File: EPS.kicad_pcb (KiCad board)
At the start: 4 copper layers, 90.2 x 95.9 mm, 197 parts, among them IC1 BQ7791514PWR, IC10 INA260AIPWR, IC12 LM74700QDBVRQ1, IC13 LM74700QDBVRQ1, IC14 LM5176PWPR, IC15 SN65HVD1782QDRQ1, IC16 TPS2121RUXR, IC17 TCAN1046AVDRQ1, IC18 INA260AIPWR, IC19 LM5060Q1MM_NOPB, IC2 INA260AIPWR, IC20 LM5060Q1MM_NOPB, IC21 MCP2517FD-H_SL, IC3 INA260AIPWR, IC4 INA260AIPWR, IC5 TPS22990DMLR, IC6 TPS22990DMLR, IC7 TPS22990DMLR, IC9 INA260AIPWR, J1 Barrel_Jack_Switch, J2 PH1RA-02-UA, J3 WJ126V-5.0-2P, J4 USB_C_Receptacle_USB2.0_16P, J6 TagConnect_TC2030-NL, Q10 BSZ067N06LS3_G, Q11 BSZ067N06LS3_G, Q12 BSZ067N06LS3_G, Q13 BSZ067N06LS3_G, Q15 BSZ067N06LS3_G, Q16 BSZ067N06LS3_G, Q5 BSZ067N06LS3_G, Q6 BSZ067N06LS3_G, Q8 BSZ067N06LS3_G, Q9 BSZ067N06LS3_G, U2 RP2354A_60QFN, Y1 ABM8AIG-20MHz-12-2Z-T3, Y2 ABM8-272-T3

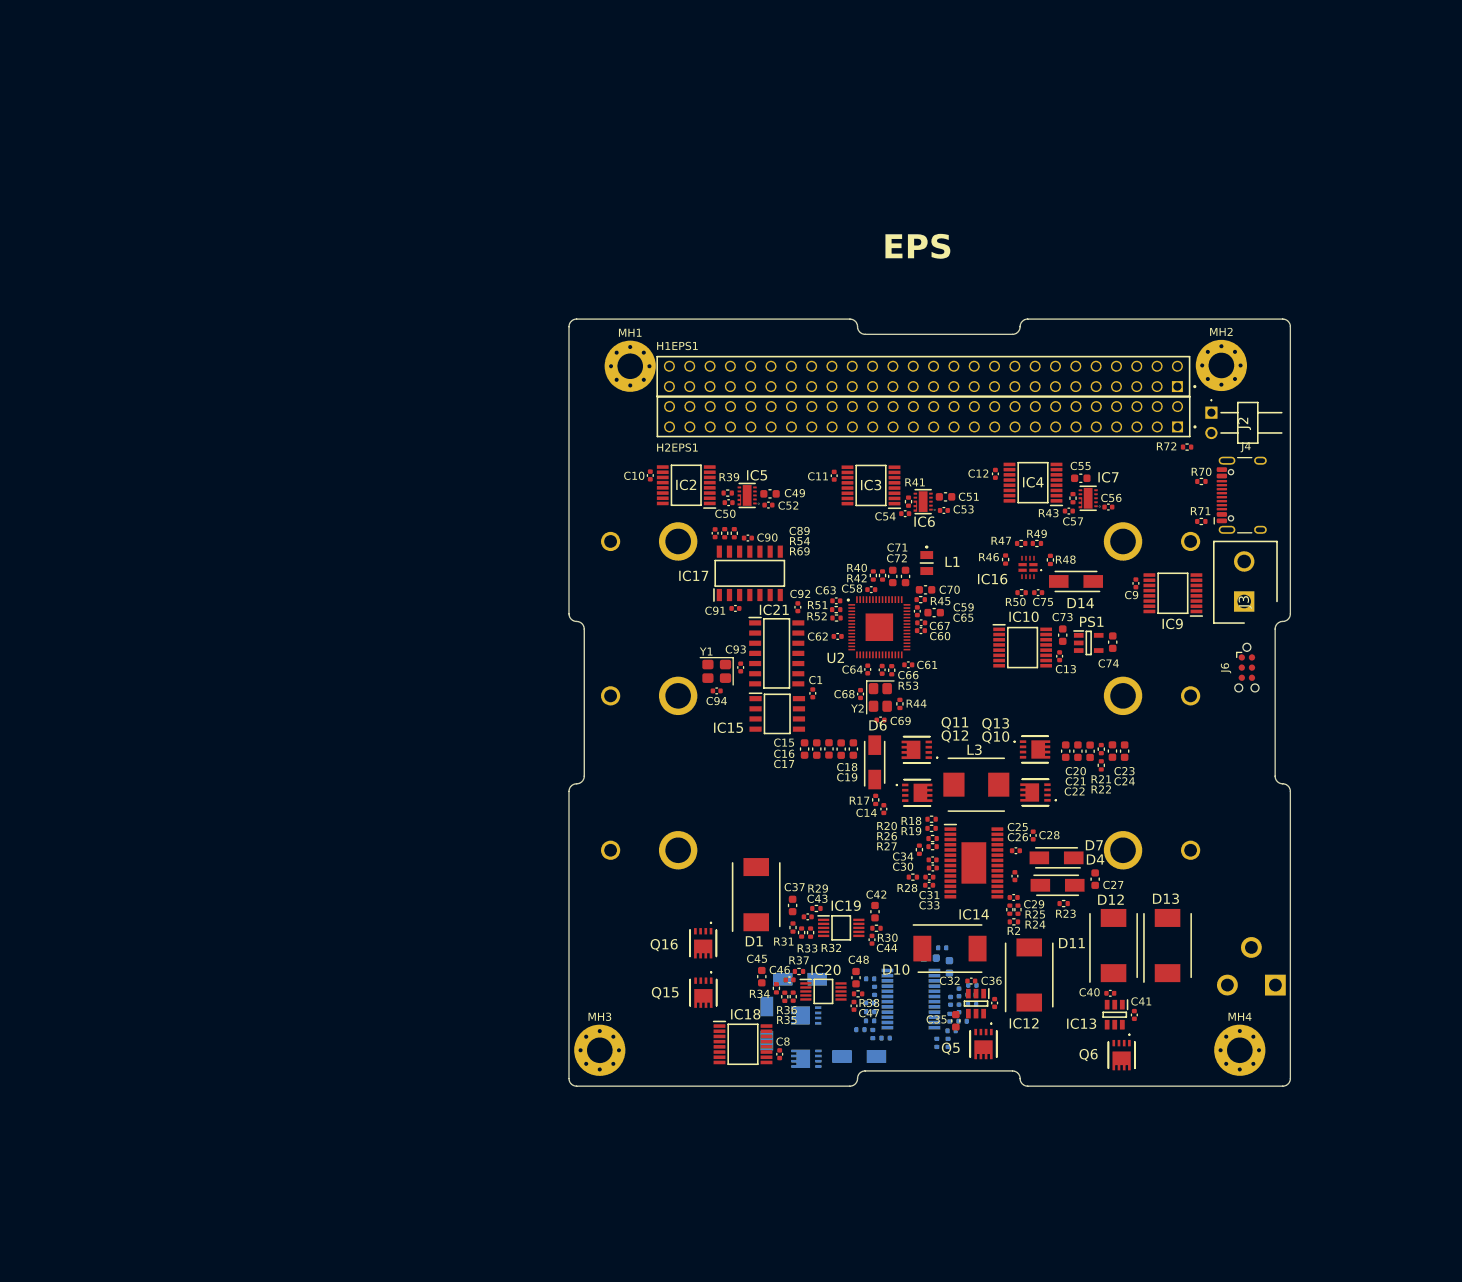
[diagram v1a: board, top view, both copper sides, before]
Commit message: Rev 1 version
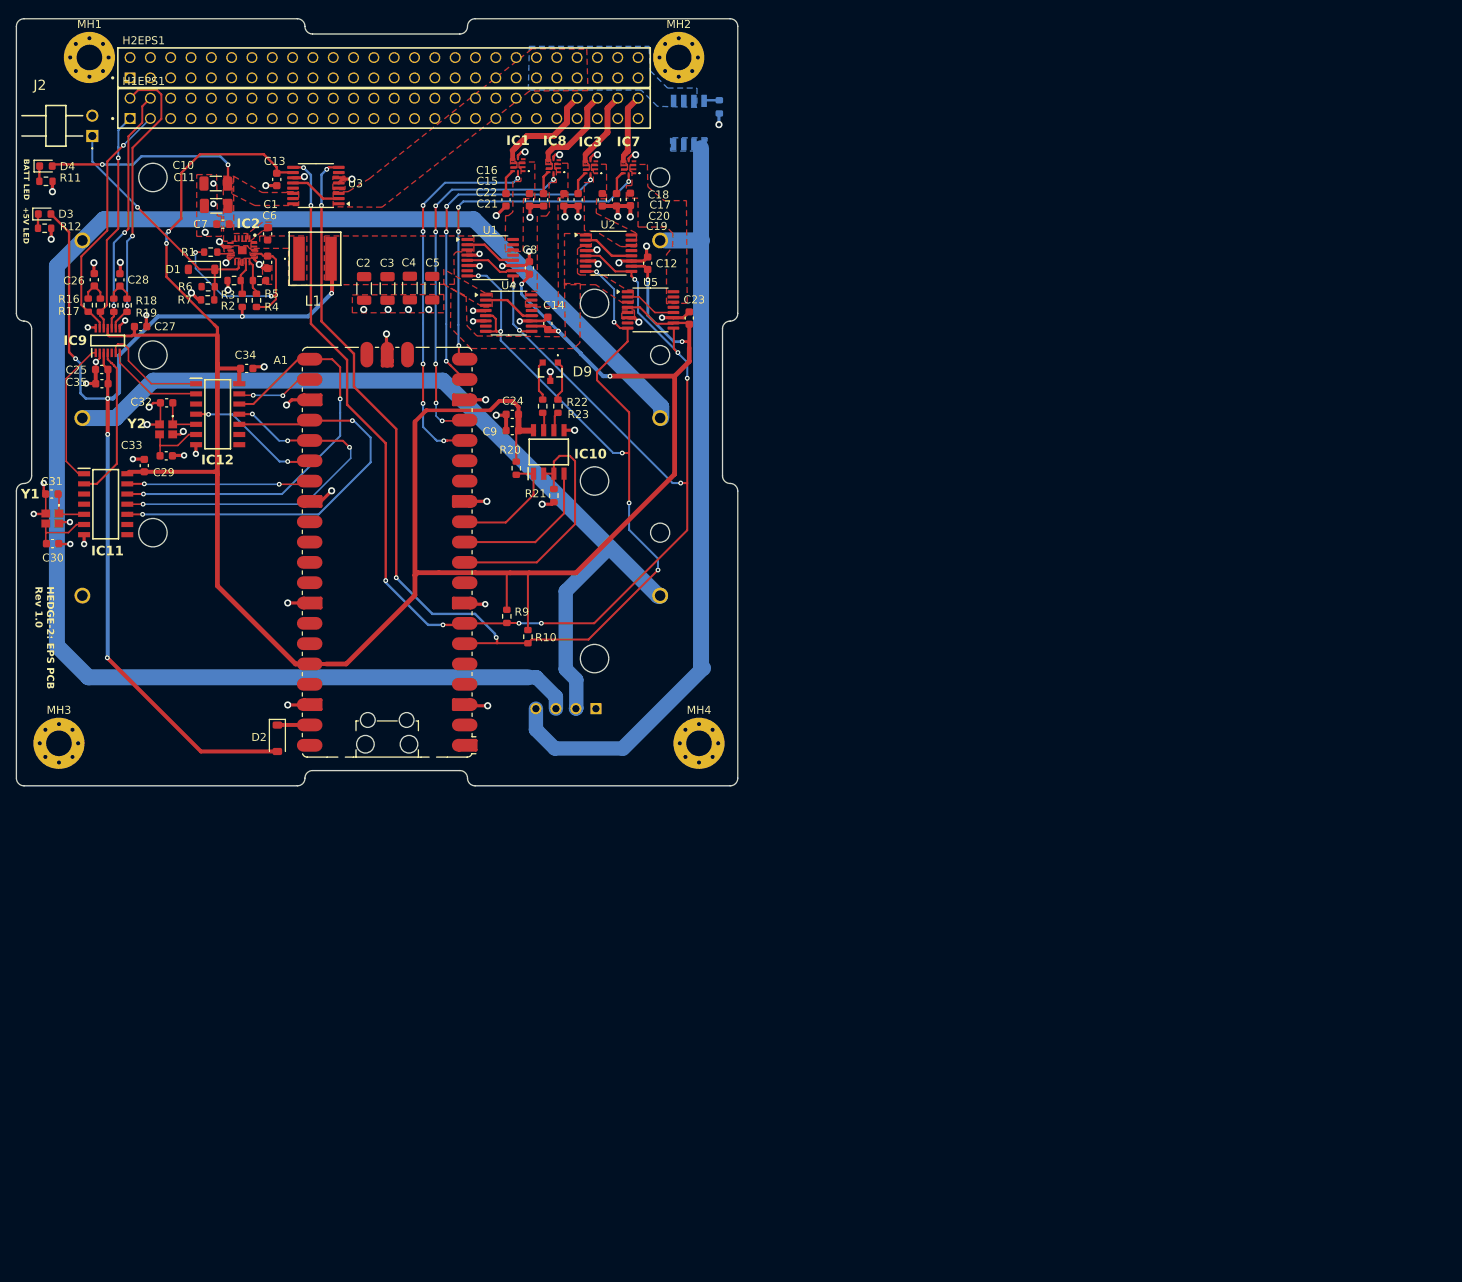
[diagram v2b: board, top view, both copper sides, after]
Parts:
- removed C36, C41, C43, C44, C46, C47, C50, C54, C57, C58, C59, C60, C61, C62, C63, C64, C66, C67, C75, C89, C90, C91, C92: 100n, Capacitor_SMD:C_0402_1005Metric
- removed C37, C42, C45, C48: 22u, Capacitor_SMD:C_0603_1608Metric
- removed C40: 22n, Capacitor_SMD:C_0402_1005Metric
- removed C49, C51, C55, C73, C74: 1u, Capacitor_SMD:C_0603_1608Metric
- removed C52, C53, C56: 220p, Capacitor_SMD:C_0402_1005Metric
- removed C65, C70, C71, C72: 4u7, Capacitor_SMD:C_0603_1608Metric
- removed C68, C69, C93, C94: 15p, Capacitor_SMD:C_0402_1005Metric
- removed D10, D11, D12, D13: SMCJ36A, HEDGE2:SMCJ36A
- removed D14, D5, D6, D7: CDBA240LL-HF, 40V 2A, HEDGE2:CDBA240LL-HF
- removed IC13: LM74700QDBVRQ1, HEDGE2:LM74700QDBVRQ1
- removed IC14: LM5176PWPR, HEDGE2:LM5176PWPR
- removed IC15: SN65HVD1782QDRQ1, HEDGE2:SN65HVD1782QDRQ1
- removed IC16: TPS2121RUXR, HEDGE2:TPS2121RUXR
- removed IC17: TCAN1046AVDRQ1, HEDGE2:TCAN1046AVDRQ1
- removed IC18, IC4: INA260AIPWR, HEDGE2:INA260AIPWR
- removed IC19, IC20: LM5060Q1MM_NOPB, HEDGE2:LM5060Q1MM_NOPB
- removed IC21: MCP2517FD-H_SL, HEDGE2:MCP2517FD-H_SL
- removed IC5, IC6: TPS22990DMLR, HEDGE2:TPS22990DMLR
- removed J3: WJ126V-5.0-2P, HEDGE2:WJ126V-5.0-2P
- removed J4: USB_C_Receptacle_USB2.0_16P, Connector_USB:USB_C_Receptacle_HCTL_HC-TYPE-C-16P-01A
- removed J6: TagConnect_TC2030-NL, Connector:Tag-Connect_TC2030-IDC-NL_2x03_P1.27mm_Vertical
- removed L3: 0630CDMCDDS-1R2MC, HEDGE2:0630CDMCDDS-1R2MC
- removed PS1: TLV75733PDBVR, HEDGE2:TLV75733PDBVR
- removed Q10, Q11, Q12, Q13, Q15, Q16, Q5, Q6, Q8, Q9: BSZ067N06LS3_G, HEDGE2:BSZ067N06LS3G
- removed R13: 450k, Resistor_SMD:R_0402_1005Metric
- removed R14, R30, R38: 100k, Resistor_SMD:R_0402_1005Metric
- removed R15, R39, R41, R43, R53, TH1: 10k, Resistor_SMD:R_0402_1005Metric
- removed R24, R25: 100, Resistor_SMD:R_0402_1005Metric
- removed R26: 93k1, Resistor_SMD:R_0402_1005Metric
- removed R27: 23k2, Resistor_SMD:R_0402_1005Metric
- removed R28: 7k5, Resistor_SMD:R_0402_1005Metric
- removed R29, R37: 9k09, Resistor_SMD:R_0402_1005Metric
- removed R31, R34: 200k, Resistor_SMD:R_0402_1005Metric
- removed R32, R35: 38k3, Resistor_SMD:R_0402_1005Metric
- removed R33, R36: 14k, Resistor_SMD:R_0402_1005Metric
- removed R40, R42: 27, Resistor_SMD:R_0402_1005Metric
- removed R44: 1k, Resistor_SMD:R_0402_1005Metric
- removed R45: 33, Resistor_SMD:R_0402_1005Metric
- removed R46, R48: 23k7, Resistor_SMD:R_0402_1005Metric
- removed R47, R49: 5k, Resistor_SMD:R_0402_1005Metric
- removed R50: 51k1, Resistor_SMD:R_0402_1005Metric
- removed R51, R52, R72: 4k7, Resistor_SMD:R_0402_1005Metric
- removed R54, R69: 60, Resistor_SMD:R_0402_1005Metric
- removed R70, R71: 5k1, Resistor_SMD:R_0402_1005Metric
- added A1: RaspberryPi_Pico, Module:RaspberryPi_Pico_SMD_HandSolder, F.Cu at (154.8, 119.7)
- added BT2: 1043, HEDGE2-EPS:BAT_1043, B.Cu at (152.8, 103.0)
- added BT3: 1043, HEDGE2-EPS:BAT_1043, B.Cu at (152.8, 80.8)
- added D9: SM712-02HTG, HEDGE2-EPS:SM71202HTG, F.Cu at (175.2, 97.2)
- added IC11: MCP2518FDT-E_SL, HEDGE2-EPS:MCP2518FDT-E_SL, F.Cu at (119.6, 113.7)
- added IC8: TPS22997RYZR, HEDGE2-EPS:TPS22997RYZR, F.Cu at (175.6, 71.5)
- added Q1: SI4497DY-T1-GE3, HEDGE2-EPS:SI4497DY-T1-GE3, B.Cu at (192.5, 66.0)
- added U1: INA260, Package_SO:TSSOP-16_4.4x5mm_P0.65mm, F.Cu at (167.7, 82.9)
- added U3: INA260, Package_SO:TSSOP-16_4.4x5mm_P0.65mm, F.Cu at (145.9, 73.9)
- added U4: INA260, Package_SO:TSSOP-16_4.4x5mm_P0.65mm, F.Cu at (170.0, 89.9)
- added U5: INA260, Package_SO:TSSOP-16_4.4x5mm_P0.65mm, F.Cu at (187.7, 89.5)
- BT1: value BK-18650-PC6 -> 1043; footprint HEDGE2:BK18650PC6 -> HEDGE2-EPS:BAT_1043
- C1, C12, C13, C14, C25, C26, C28, C8, C9: footprint Capacitor_SMD:C_0402_1005Metric -> Capacitor_SMD:C_0603_1608Metric
- C10, C11: value 100n -> 22u; footprint Capacitor_SMD:C_0402_1005Metric -> Capacitor_SMD:C_1206_3216Metric
- C15, C17: value 33u -> 100n
- C16: value 33u -> 1n
- C18: value 10u -> 1n
- C19: value 10u -> 100n
- C2, C3: value 1u -> 47u; footprint Capacitor_SMD:C_0603_1608Metric -> Capacitor_SMD:C_1206_3216Metric; moved to F.Cu
- C20, C22: value 22u -> 1n
- C21: value 22u -> 100n
- C23, C24: value 220u -> 100n
- C27: value 1u -> 100n
- C29: value 47p -> 100n; footprint Capacitor_SMD:C_0402_1005Metric -> Capacitor_SMD:C_0603_1608Metric
- C30, C31: value 15n -> 10p; footprint Capacitor_SMD:C_0402_1005Metric -> Capacitor_SMD:C_0603_1608Metric
- C32: value 22n -> 10p; footprint Capacitor_SMD:C_0402_1005Metric -> Capacitor_SMD:C_0603_1608Metric
- C33: value 180p -> 10p; footprint Capacitor_SMD:C_0402_1005Metric -> Capacitor_SMD:C_0603_1608Metric
- C34: value 100p -> 100n; footprint Capacitor_SMD:C_0402_1005Metric -> Capacitor_SMD:C_0603_1608Metric
- C35: value 47u -> 10uF
- C4, C5: value 100n -> 47u; footprint Capacitor_SMD:C_0402_1005Metric -> Capacitor_SMD:C_1206_3216Metric; moved to F.Cu
- C6, C7: footprint Capacitor_SMD:C_0402_1005Metric -> Capacitor_SMD:C_0603_1608Metric; moved to F.Cu
- D1: value SMCJ36A -> Zener; footprint HEDGE2:SMCJ36A -> Diode_SMD:D_SOD-123
- D2: value CDBA240LL-HF, 40V 2A -> Schottky; footprint HEDGE2:CDBA240LL-HF -> Diode_SMD:D_SOD-123; moved to F.Cu
- D3: value CDBA240LL-HF, 40V 2A -> LED; footprint HEDGE2:CDBA240LL-HF -> LED_SMD:LED_0603_1608Metric; moved to F.Cu
- D4: value CDBA240LL-HF, 40V 2A -> LED; footprint HEDGE2:CDBA240LL-HF -> LED_SMD:LED_0603_1608Metric
- H1EPS1, H2EPS1: footprint HEDGE2:SAMTEC_ESQ-126-39-G-D -> HEDGE2-EPS:SAMTEC_ESQ-126-39-G-D
- IC1: value BQ7791514PWR -> TPS22997RYZR; footprint HEDGE2:BQ7791501PWR -> HEDGE2-EPS:TPS22997RYZR; moved to F.Cu
- IC10: value INA260AIPWR -> SN65HVD1782QDRQ1; footprint HEDGE2:INA260AIPWR -> HEDGE2-EPS:SN65HVD1782QDRQ1
- IC12: value LM74700QDBVRQ1 -> MCP2518FDT-E_SL; footprint HEDGE2:LM74700QDBVRQ1 -> HEDGE2-EPS:MCP2518FDT-E_SL
- IC2: value INA260AIPWR -> TPS56C230RJER; footprint HEDGE2:INA260AIPWR -> HEDGE2-EPS:TPS56C230RJER
- IC3: value INA260AIPWR -> TPS22997RYZR; footprint HEDGE2:INA260AIPWR -> HEDGE2-EPS:TPS22997RYZR
- IC7: value TPS22990DMLR -> TPS22997RYZR; footprint HEDGE2:TPS22990DMLR -> HEDGE2-EPS:TPS22997RYZR
- IC9: value INA260AIPWR -> TCAN1046AVDYYRQ1; footprint HEDGE2:INA260AIPWR -> HEDGE2-EPS:TCAN1046AVDYYRQ1
- J1: value Barrel_Jack_Switch -> S4B-XH-A_LF__SN_; footprint Connector_BarrelJack:BarrelJack_CUI_PJ-102AH_Horizontal -> HEDGE2-EPS:S4BXHALFSN
- J2: footprint HEDGE2:PH1RA02UA -> HEDGE2-EPS:PH1RA02UA
- L1: value 3u3 AOTA-B201610S3R3-101-T -> 3u3; footprint HEDGE2:AOTAB201610S3R3101T -> HEDGE2-EPS:744393465033
- R1: value 1k -> 100k; footprint Resistor_SMD:R_0402_1005Metric -> Resistor_SMD:R_0603_1608Metric; moved to F.Cu
- R10, R11, R9: value 1M -> 4k7; footprint Resistor_SMD:R_0402_1005Metric -> Resistor_SMD:R_0603_1608Metric; moved to F.Cu
- R12: value 3M3 -> 2k2; footprint Resistor_SMD:R_0402_1005Metric -> Resistor_SMD:R_0603_1608Metric; moved to F.Cu
- R16: value 10k -> 60; footprint Resistor_SMD:R_0402_1005Metric -> Resistor_SMD:R_0603_1608Metric; moved to F.Cu
- R17: value 10 -> 60; footprint Resistor_SMD:R_0402_1005Metric -> Resistor_SMD:R_0603_1608Metric
- R18: value 249k -> 60; footprint Resistor_SMD:R_0402_1005Metric -> Resistor_SMD:R_0603_1608Metric
- R19: value 71k5 -> 60; footprint Resistor_SMD:R_0402_1005Metric -> Resistor_SMD:R_0603_1608Metric
- R2: value 9m -> 110k; footprint Resistor_SMD:R_0402_1005Metric -> Resistor_SMD:R_0603_1608Metric
- R20: value 2k -> 10k; footprint Resistor_SMD:R_0402_1005Metric -> Resistor_SMD:R_0603_1608Metric
- R21: value 105k -> 10k; footprint Resistor_SMD:R_0402_1005Metric -> Resistor_SMD:R_0603_1608Metric
- R22: value 20k -> 10; footprint Resistor_SMD:R_0402_1005Metric -> Resistor_SMD:R_0603_1608Metric
- R23: value 10k -> 10; footprint Resistor_SMD:R_0402_1005Metric -> Resistor_SMD:R_0603_1608Metric
- R3: value 1k -> 15k; footprint Resistor_SMD:R_0402_1005Metric -> Resistor_SMD:R_0603_1608Metric; moved to F.Cu
- R4: value 1k -> 180k; footprint Resistor_SMD:R_0402_1005Metric -> Resistor_SMD:R_0603_1608Metric; moved to F.Cu
- R5: value 1k -> 33k; footprint Resistor_SMD:R_0402_1005Metric -> Resistor_SMD:R_0603_1608Metric; moved to F.Cu
- R6: value 1k -> 205k; footprint Resistor_SMD:R_0402_1005Metric -> Resistor_SMD:R_0603_1608Metric; moved to F.Cu
- R7: value 10m -> 51k1; footprint Resistor_SMD:R_0402_1005Metric -> Resistor_SMD:R_0603_1608Metric; moved to F.Cu
- R8: value 4k5 -> 10k; footprint Resistor_SMD:R_0402_1005Metric -> Resistor_SMD:R_0603_1608Metric
- U2: value RP2354A_60QFN -> INA260; footprint HEDGE2:RP2354A -> Package_SO:TSSOP-16_4.4x5mm_P0.65mm
- Y1: value ABM8AIG-20MHz-12-2Z-T3 -> 40MHz; footprint Crystal:Crystal_SMD_3225-4Pin_3.2x2.5mm -> HEDGE2-EPS:ABM10AIG-40.000MHZ-7-J1Z-T
- Y2: value ABM8-272-T3 -> 40MHz; footprint Crystal:Crystal_SMD_3225-4Pin_3.2x2.5mm -> HEDGE2-EPS:ABM10AIG-40.000MHZ-7-J1Z-T
- moved D4 155.2 mm to (112.2, 71.5)
- moved R11 148.5 mm to (112.2, 73.4), turned to 0 degrees
- moved J2 144.1 mm to (118.0, 67.7), turned to 90 degrees
- moved R12 142.9 mm to (112.0, 79.2)
- moved H2EPS1 138.0 mm to (122.7, 60.4)
- moved C27 137.9 mm to (124.0, 91.5), turned to 0 degrees
- moved C26 137.1 mm to (118.2, 85.7), turned to 90 degrees
- moved IC9 136.8 mm to (119.9, 93.3), turned to 90 degrees
- moved H1EPS1 135.1 mm to (122.7, 65.5)
- moved C7 134.5 mm to (134.3, 78.7), turned to 180 degrees
- moved D3 134.4 mm to (112.0, 77.5)
- moved C28 133.6 mm to (121.4, 85.7), turned to 90 degrees
- moved C35 133.2 mm to (119.2, 98.7), turned to 180 degrees
- moved R6 131.6 mm to (132.4, 86.5), turned to 0 degrees
- moved R16 130.4 mm to (117.4, 88.9)
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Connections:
- net /UART_E_RX renamed /UART_E_RX (SCI)
- net /UART_E_TX renamed /UART_E_TX (SCI)
- net /UART_F_RX renamed /UART_F_RX (GNSS_RXD1)
- net /UART_F_TX renamed /UART_F_TX (GNSS_TXD1)
- C1 pad 1: 3V3 -> Net-(IC2-BST)
- C1 pad 2: GND -> Net-(IC2-SW_1)
- C10 pad 1: +3V3 -> +BATT_SENSE
- C11 pad 1: +3V3 -> +BATT_SENSE
- C14 pad 1: Net-(IC14-VIN) -> +3V3
- C15 pad 1: +BUCK_BOOST -> +5V_OBC_SENSE
- C16 pad 1: +BUCK_BOOST -> Net-(IC1-CT)
- C17 pad 1: +BUCK_BOOST -> +5V_SCI_SENSE
- C18 pad 1: +BUCK_BOOST -> Net-(IC3-CT)
- C19 pad 1: +BUCK_BOOST -> +5V_COMM_SENSE
- C2 pad 1: Net-(IC1-VDD) -> +5V
- C20 pad 1: +5V_BUCK_BOOST -> Net-(IC7-CT)
- C21 pad 1: +5V_BUCK_BOOST -> +5V_GNSS_SENSE
- C22 pad 1: +5V_BUCK_BOOST -> Net-(IC8-CT)
- C23 pad 1: +5V_BUCK_BOOST -> +3V3
- C24 pad 1: +5V_BUCK_BOOST -> +3V3
- C25 pad 1: /Power Conversion/BIAS -> +5V
- C26 pad 1: Net-(D4-K) -> Net-(C26-Pad1)
- C26 pad 2: /Power Conversion/SW2 -> GND
- C27 pad 1: /Power Conversion/VCC -> +3V3
- C28 pad 1: /Power Conversion/SW1 -> Net-(C28-Pad1)
- C28 pad 2: Net-(D7-K) -> GND
- C29 pad 1: Net-(IC14-CSG) -> +3V3
- C29 pad 2: Net-(IC14-CS) -> GND
- C3 pad 1: GND -> +5V
- C3 pad 2: Net-(IC1-AVDD) -> GND
- C30 pad 1: Net-(IC14-SS) -> Net-(IC11-OSC1)
- C31 pad 1: Net-(IC14-COMP) -> Net-(IC11-OSC2)
- C31 pad 2: Net-(C31-Pad2) -> GND
- C32 pad 1: -BATT_IN -> Net-(IC12-OSC2)
- C33 pad 1: Net-(IC14-COMP) -> Net-(IC12-OSC1)
- C34 pad 1: Net-(IC14-SLOPE) -> +3V3
- C35 pad 1: +BUCK_BOOST -> +5V
- C4 pad 1: Net-(IC1-VC3) -> +5V
- C4 pad 2: Net-(IC1-VC2) -> GND
- C5 pad 1: Net-(IC1-VC2) -> +5V
- C5 pad 2: Net-(IC1-VC1) -> GND
- C6 pad 1: Net-(IC1-VC1) -> Net-(IC2-VCC)
- C7 pad 1: GND -> +BATT_SENSE
- C7 pad 2: Net-(IC1-VC0) -> GND
- D1 pad 1: +BATT -> /EN
- D2 pad 1: Net-(D2-K) -> Net-(A1-VSYS)
- D2 pad 2: Net-(D2-A) -> +5V
- D3 pad 2: PACK- -> +5V
- D4 pad 2: /Power Conversion/VCC -> +BATT_SENSE
- H1EPS1 pad 05: /UART_A_TX -> unconnected-(H1EPS1-Pad05)
- H1EPS1 pad 06: /UART_B_TX -> unconnected-(H1EPS1-Pad06)
- H1EPS1 pad 07: /UART_A_RX -> unconnected-(H1EPS1-Pad07)
- H1EPS1 pad 08: /UART_B_RX -> unconnected-(H1EPS1-Pad08)
- H1EPS1 pad 13: /UART_C_TX -> unconnected-(H1EPS1-Pad13)
- H1EPS1 pad 15: /UART_C_RX -> unconnected-(H1EPS1-Pad15)
- H1EPS1 pad 22: /UART_D_TX -> unconnected-(H1EPS1-Pad22)
- H1EPS1 pad 24: /UART_D_RX -> unconnected-(H1EPS1-Pad24)
- H1EPS1 pad 25: /5V_PERM -> unconnected-(H1EPS1-Pad25)
- H1EPS1 pad 26: /5V_PERM -> unconnected-(H1EPS1-Pad26)
- H1EPS1 pad 29: GND -> unconnected-(H1EPS1-Pad29)
- H1EPS1 pad 30: GND -> unconnected-(H1EPS1-Pad30)
- H1EPS1 pad 31: GND -> unconnected-(H1EPS1-Pad31)
- H1EPS1 pad 32: GND -> unconnected-(H1EPS1-Pad32)
- H1EPS1 pad 33: unconnected-(H1EPS1-Pad33) -> GND
- H1EPS1 pad 34: unconnected-(H1EPS1-Pad34) -> GND
- H1EPS1 pad 41: unconnected-(H1EPS1-Pad41) -> /UART_G_TX (EPS)
- H1EPS1 pad 43: unconnected-(H1EPS1-Pad43) -> /UART_G_RX (EPS)
- H1EPS1 pad 45: /ENA_PWR_1 -> unconnected-(H1EPS1-Pad45)
- H1EPS1 pad 46: /PWR_1 -> +5V_OBC
- H1EPS1 pad 47: /ENA_PWR_2 -> unconnected-(H1EPS1-Pad47)
- H1EPS1 pad 48: /PWR_2 -> +5V_GNSS
- H1EPS1 pad 49: /ENA_PWR_3 -> unconnected-(H1EPS1-Pad49)
- H1EPS1 pad 50: /PWR_3 -> +5V_SCI
- H1EPS1 pad 51: /ENA_PWR_4 -> unconnected-(H1EPS1-Pad51)
- H1EPS1 pad 52: /PWR_4 -> +5V_COMM
- H2EPS1 pad 01: unconnected-(H2EPS1-Pad01) -> /DIN/CONFIG/DIO14_XB
- H2EPS1 pad 02: unconnected-(H2EPS1-Pad02) -> /DOUT/DIO13_XB
- H2EPS1 pad 03: unconnected-(H2EPS1-Pad03) -> /RTS/DIO6_XB
- H2EPS1 pad 04: unconnected-(H2EPS1-Pad04) -> /CTS/DIO7_XB
- H2EPS1 pad 05: unconnected-(H2EPS1-Pad05) -> /AD3/DIO3/SPI_SSEL_XB
- H2EPS1 pad 06: unconnected-(H2EPS1-Pad06) -> /AD/DIO2/SPI_CLK_XB
- H2EPS1 pad 07: unconnected-(H2EPS1-Pad07) -> /DIO4/SPI_MOSI_XB
- H2EPS1 pad 08: unconnected-(H2EPS1-Pad08) -> /DIO12/SPI_MISO_XB
- H2EPS1 pad 09: unconnected-(H2EPS1-Pad09) -> /DTR/SLEEP_RQ/DIO8_XB
- H2EPS1 pad 10: unconnected-(H2EPS1-Pad10) -> /AD1/DIO1/SPI_ATTN_XB
- H2EPS1 pad 11: unconnected-(H2EPS1-Pad11) -> /ON_SLEEP/DIO9_XB
- H2EPS1 pad 12: unconnected-(H2EPS1-Pad12) -> /DIO10/PWM0_XB
- H2EPS1 pad 13: unconnected-(H2EPS1-Pad13) -> /RESET_XB
- H2EPS1 pad 14: unconnected-(H2EPS1-Pad14) -> /DIO11/PWM1_XB
- H2EPS1 pad 15: unconnected-(H2EPS1-Pad15) -> /AD0/DIO0_XB
- H2EPS1 pad 16: unconnected-(H2EPS1-Pad16) -> /Associate/DIO5_XB
- H2EPS1 pad 17: unconnected-(H2EPS1-Pad17) -> /NDTR_XB
- H2EPS1 pad 19: unconnected-(H2EPS1-Pad19) -> /MIC_IN_DMR
- H2EPS1 pad 20: unconnected-(H2EPS1-Pad20) -> /LINE_OUT_DMR
- H2EPS1 pad 21: unconnected-(H2EPS1-Pad21) -> /T/R_DMR
- H2EPS1 pad 22: unconnected-(H2EPS1-Pad22) -> /PTT_DMR
- H2EPS1 pad 23: unconnected-(H2EPS1-Pad23) -> /SPKEN_DMR
- H2EPS1 pad 24: unconnected-(H2EPS1-Pad24) -> /CS_DMR
- H2EPS1 pad 25: /5V_PERM -> /HST_RXD_DMR
- H2EPS1 pad 26: /5V_PERM -> /UART_RX_DMR
- H2EPS1 pad 27: unconnected-(H2EPS1-Pad27) -> /HST_TXD_DMR
- H2EPS1 pad 28: unconnected-(H2EPS1-Pad28) -> /UART_TX_DMR
- H2EPS1 pad 33: /ENA_PWR_5 -> unconnected-(H2EPS1-Pad33)
- H2EPS1 pad 34: /PWR_5 -> unconnected-(H2EPS1-Pad34)
- H2EPS1 pad 35: /ENA_PWR_6 -> unconnected-(H2EPS1-Pad35)
- H2EPS1 pad 36: /PWR_6 -> unconnected-(H2EPS1-Pad36)
- H2EPS1 pad 37: /ENA_PWR_7 -> unconnected-(H2EPS1-Pad37)
- H2EPS1 pad 38: /PWR_7 -> unconnected-(H2EPS1-Pad38)
- H2EPS1 pad 39: /ENA_PWR_8 -> unconnected-(H2EPS1-Pad39)
- H2EPS1 pad 40: /PWR_8 -> unconnected-(H2EPS1-Pad40)
- H2EPS1 pad 41: unconnected-(H2EPS1-Pad41) -> BATT
- H2EPS1 pad 42: unconnected-(H2EPS1-Pad42) -> BATT
- H2EPS1 pad 43: /CHARGE -> BATT
- H2EPS1 pad 44: /CHARGE -> BATT
- H2EPS1 pad 45: /BATT -> BATT
- H2EPS1 pad 46: /BATT -> BATT
- H2EPS1 pad 47: /RBF_A -> unconnected-(H2EPS1-Pad47)
- H2EPS1 pad 48: /DS_A -> unconnected-(H2EPS1-Pad48)
- H2EPS1 pad 49: /RBF_B -> unconnected-(H2EPS1-Pad49)
- H2EPS1 pad 50: /DS_B -> unconnected-(H2EPS1-Pad50)
- H2EPS1 pad 51: /RBF_C -> unconnected-(H2EPS1-Pad51)
- H2EPS1 pad 52: /DS_C -> unconnected-(H2EPS1-Pad52)
- IC1 pad 1: Net-(IC1-VDD) -> +5V_OBC_SENSE
- IC1 pad 10: GND -> /OBC_C
- IC1 pad 2: Net-(IC1-AVDD) -> +5V_OBC_SENSE
- IC1 pad 3: Net-(IC1-VC3) -> +5V_OBC_SENSE
- IC1 pad 4: Net-(IC1-VC3) -> unconnected-(IC1-PG-Pad4)
- IC1 pad 5: Net-(IC1-VC3) -> GND
- IC1 pad 6: Net-(IC1-VC2) -> +5V_OBC
- IC1 pad 7: Net-(IC1-VC1) -> +5V_OBC
- IC1 pad 8: Net-(IC1-VC0) -> +5V_OBC
- IC1 pad 9: GND -> Net-(IC1-CT)
- IC10 pad 1: +EPS_5V -> /RS485_RX
- IC10 pad 2: +EPS_5V -> /RS485_E
- IC10 pad 3: +EPS_5V -> /RS485_E
- IC10 pad 4: +3V3 -> /RS485_TX
- IC10 pad 5: SDA -> GND
- IC10 pad 6: GND -> Net-(IC10-A)
- IC10 pad 7: unconnected-(IC10-ALERT-Pad7) -> Net-(IC10-B)
- IC10 pad 8: SDA -> +3V3
- IC12 pad 1: Net-(IC12-VCAP) -> /TXCAN_B
- IC12 pad 2: GND -> /RXCAN_B
- IC12 pad 3: -BATT_IN -> unconnected-(IC12-CLKO/SOF-Pad3)
- IC12 pad 4: +BUCK_BOOST -> /CAN_B_INT
- IC12 pad 5: Net-(IC12-GATE) -> Net-(IC12-OSC2)
- IC12 pad 6: -BATT_IN -> Net-(IC12-OSC1)
- IC2 pad 1: +5V_OBC_IN -> Net-(IC2-BST)
- IC2 pad 10: +3V3 -> GND
- IC2 pad 11: GND -> unconnected-(IC2-SS-Pad11)
- IC2 pad 12: +5V_OBC_IN -> /EN
- IC2 pad 13: unconnected-(IC2-NC-Pad13) -> GND
- IC2 pad 14: -5V_OBC_IN -> Net-(IC2-FB)
- IC2 pad 15: -5V_OBC_IN -> Net-(IC2-MODE)
- IC2 pad 16: -5V_OBC_IN -> GND
- IC2 pad 2: +5V_OBC_IN -> +BATT_SENSE
- IC2 pad 3: +5V_OBC_IN -> +BATT_SENSE
- IC2 pad 4: GND -> +BATT_SENSE
- IC2 pad 5: SCL -> +BATT_SENSE
- IC2 pad 6: GND -> Net-(IC2-SW_1)
- IC2 pad 7: unconnected-(IC2-ALERT-Pad7) -> GND
- IC2 pad 8: SDA -> GND
- IC2 pad 9: SCL -> Net-(IC2-PGOOD)
- IC3 pad 1: +COMMS_IN -> +5V_SCI_SENSE
- IC3 pad 10: +3V3 -> /SCI_C
- IC3 pad 2: +COMMS_IN -> +5V_SCI_SENSE
- IC3 pad 3: +COMMS_IN -> +5V_SCI_SENSE
- IC3 pad 4: +3V3 -> unconnected-(IC3-PG-Pad4)
- IC3 pad 6: GND -> +5V_SCI
- IC3 pad 7: unconnected-(IC3-ALERT-Pad7) -> +5V_SCI
- IC3 pad 8: SDA -> +5V_SCI
- IC3 pad 9: SCL -> Net-(IC3-CT)
- IC7 pad 1: Net-(IC7-CT) -> +5V_COMM_SENSE
- IC7 pad 10: +SCI_IN -> /COMM_C
- IC7 pad 2: unconnected-(IC7-NC-Pad2) -> +5V_COMM_SENSE
- IC7 pad 3: +5V_BUCK_BOOST -> +5V_COMM_SENSE
- IC7 pad 4: +5V_BUCK_BOOST -> unconnected-(IC7-PG-Pad4)
- IC7 pad 5: SCI_EN -> GND
- IC7 pad 6: GND -> +5V_COMM
- IC7 pad 7: Net-(IC7-PG) -> +5V_COMM
- IC7 pad 8: +SCI_IN -> +5V_COMM
- IC7 pad 9: +SCI_IN -> Net-(IC7-CT)
- IC9 pad 1: +BENCH_IN -> /TXCAN_A
- IC9 pad 10: +3V3 -> /CAN_B_H
- IC9 pad 11: GND -> +3V3
- IC9 pad 12: +BENCH_IN -> /CAN_A_L
- IC9 pad 13: unconnected-(IC9-NC-Pad13) -> /CAN_A_H
- IC9 pad 14: -BENCH_IN -> GND
- IC9 pad 2: +BENCH_IN -> GND
- IC9 pad 3: +BENCH_IN -> +5V
- IC9 pad 4: GND -> /RXCAN_A
- IC9 pad 5: SDA -> GND
- IC9 pad 6: GND -> /TXCAN_B
- IC9 pad 7: unconnected-(IC9-ALERT-Pad7) -> /RXCAN_B
- IC9 pad 8: SDA -> GND
- IC9 pad 9: SCL -> /CAN_B_L
- J1 pad 1: +BATT -> GND
- J1 pad 2: PACK- -> /VC1
- J1 pad 3: unconnected-(J1-Pad3) -> /VC2
- J2 pad 1: /RBF_INHIBIT -> /EN
- L1 pad 1: 1V1 -> Net-(IC2-SW_1)
- L1 pad 2: Net-(U2-VREG_LX) -> +5V
- R1 pad 1: +BATT -> Net-(IC2-PGOOD)
- R1 pad 2: Net-(IC1-VDD) -> Net-(IC2-VCC)
- R10 pad 1: Net-(D2-A) -> +3V3
- R10 pad 2: Net-(IC1-CHG) -> /SDA
- R11 pad 1: Net-(D2-K) -> Net-(D4-K)
- R11 pad 2: Net-(D2-A) -> GND
- R12 pad 1: PACK- -> Net-(D3-K)
- R12 pad 2: Net-(D2-K) -> GND
- R16 pad 1: Net-(IC1-VTB) -> /CAN_A_H
- R16 pad 2: GND -> Net-(C26-Pad1)
- R17 pad 1: Net-(IC14-VIN) -> Net-(C26-Pad1)
- R17 pad 2: Net-(D6-K) -> /CAN_A_L
- R18 pad 1: Net-(IC14-EN/UVLO) -> /CAN_B_H
- R18 pad 2: +BUCK_BOOST -> Net-(C28-Pad1)
- R19 pad 1: GND -> Net-(C28-Pad1)
- R19 pad 2: Net-(IC14-EN/UVLO) -> /CAN_B_L
- R2 pad 1: /Power Conversion/RCS -> +5V
- R2 pad 2: GND -> Net-(IC2-FB)
- R20 pad 1: Net-(IC14-VISNS) -> +3V3
- R20 pad 2: +BUCK_BOOST -> /RS485_RX
- R21 pad 1: +5V_BUCK_BOOST -> /RS485_E
- R21 pad 2: /Power Conversion/FB -> GND
- R22 pad 1: /Power Conversion/FB -> Net-(IC10-B)
- R22 pad 2: GND -> /UART_G_TX (EPS)
- R23 pad 1: /Power Conversion/VCC -> Net-(IC10-A)
- R23 pad 2: Net-(IC14-PGOOD) -> /UART_G_RX (EPS)
- R3 pad 1: +BATT -> Net-(IC2-FB)
- R3 pad 2: Net-(IC1-VC3) -> GND
- R4 pad 1: /Batteries/VC2 -> Net-(IC2-VCC)
- R4 pad 2: Net-(IC1-VC2) -> Net-(IC2-MODE)
- R5 pad 1: /Batteries/VC1 -> Net-(IC2-MODE)
- R5 pad 2: Net-(IC1-VC1) -> GND
- R6 pad 1: GND -> +BATT_SENSE
- R6 pad 2: Net-(IC1-VC0) -> /EN
- R7 pad 1: GND -> /EN
- R7 pad 2: Net-(D5-A) -> GND
- R8 pad 1: Net-(Q8-G) -> GND
- R8 pad 2: Net-(IC1-DSG) -> Net-(Q1-G)
- R9 pad 1: Net-(D5-A) -> +3V3
- R9 pad 2: Net-(Q8-G) -> /SCL
- U2 pad 1: 3V3 -> +5V
- U2 pad 10: STATUS1 -> +3V3
- U2 pad 11: 3V3 -> GND
- U2 pad 12: STATUS2 -> +5V
- U2 pad 13: OBC_EN -> unconnected-(U2-NC-Pad13)
- U2 pad 14: COMM_EN -> +5V_SCI_SENSE
- U2 pad 15: SCI_EN -> +5V_SCI_SENSE
- U2 pad 16: unconnected-(U2-GPIO12-Pad16) -> +5V_SCI_SENSE
- U2 pad 2: unconnected-(U2-GPIO0-Pad2) -> +5V
- U2 pad 3: Net-(U2-GPIO1) -> +5V
- U2 pad 4: Net-(U2-GPIO2) -> GND
- U2 pad 5: unconnected-(U2-GPIO3-Pad5) -> /SCL
- U2 pad 6: 1V1 -> GND
- U2 pad 8: BOUNCEBATT -> /SDA
- U2 pad 9: BATTEN -> /SCL
- Y1 pad 1: Net-(C93-Pad2) -> Net-(IC11-OSC2)
- Y1 pad 3: Net-(IC21-OSC1) -> Net-(IC11-OSC1)
- Y2 pad 1: Net-(U2-XIN) -> Net-(IC12-OSC2)
- Y2 pad 3: Net-(C69-Pad2) -> Net-(IC12-OSC1)
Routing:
- net +3V3: track 0.00 -> 312.8 mm, vias 0 -> 7
- net /VC2: track 0.00 -> 203.1 mm
- net /SDA: track 0.00 -> 185.1 mm, vias 0 -> 11
- net /SCL: track 0.00 -> 185.1 mm, vias 0 -> 12
- net +5V: track 0.00 -> 160.0 mm, vias 0 -> 6
- net GND: track 0.00 -> 133.6 mm, vias 0 -> 73
- net /VC1: track 0.00 -> 108.3 mm
- net +BATT_NP: track 0.00 -> 97.9 mm
- net /SCK: track 0.00 -> 54.0 mm, vias 0 -> 2
- net /MISO: track 0.00 -> 53.6 mm, vias 0 -> 2
- net /OBC_C: track 0.00 -> 47.9 mm, vias 0 -> 6
- net /MOSI: track 0.00 -> 47.7 mm, vias 0 -> 4
- net /GNSS_C: track 0.00 -> 47.0 mm, vias 0 -> 6
- net /COMM_C: track 0.00 -> 42.9 mm, vias 0 -> 4
- net /SCI_C: track 0.00 -> 42.7 mm, vias 0 -> 4
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- added copper zone on F.Cu, net +5V
- added copper zone on F.Cu, net +5V_COMM
- added copper zone on F.Cu, net +5V_COMM_SENSE
- added copper zone on F.Cu, net +5V_GNSS
- added copper zone on F.Cu, net +5V_GNSS_SENSE
- added copper zone on F.Cu, net +5V_OBC
- added copper zone on F.Cu, net +5V_OBC_SENSE
- added copper zone on F.Cu, net +5V_SCI
- added copper zone on F.Cu, net +5V_SCI_SENSE
- added copper zone on B.Cu, net +BATT_NP
- added copper zone on F.Cu, net +BATT_SENSE
- added copper zone on B.Cu, net BATT
- added copper zone on F.Cu, net BATT
- added copper zone on F.Cu, net GND
- added copper zone on In1.Cu, net GND
- added copper zone on In2.Cu, net GND
- added copper zone on F.Cu, net Net-(IC2-BST)
- added copper zone on F.Cu, net Net-(IC2-SW_1)
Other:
- board text added: "${REFERENCE}"
- board text added: "+5V LED"
- board text added: "BATT LED"
- board text added: "HEDGE-2: EPS PCB Rev 1.0"
- board text removed: "EPS"
